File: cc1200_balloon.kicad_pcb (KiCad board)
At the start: 4 copper layers, 50 x 30 mm, 103 parts, among them J101 BATT pads, J201 LoRa ANT pads, J202 SWD+DBG pads, J301 434MHz ANT pads, J401 GNSS ANT, J501 BMV080, Q101 DMG3401LSN-7, U201 Wio-E5, U301 CC1200, U401 AT6558R-5N32, U501 SCD40-D-R2, U502 AS3935-BQFT, U503 BME688, U504 BME688, X301 40MHz, X401 TCXO 26MHz, X402 32.768kHz

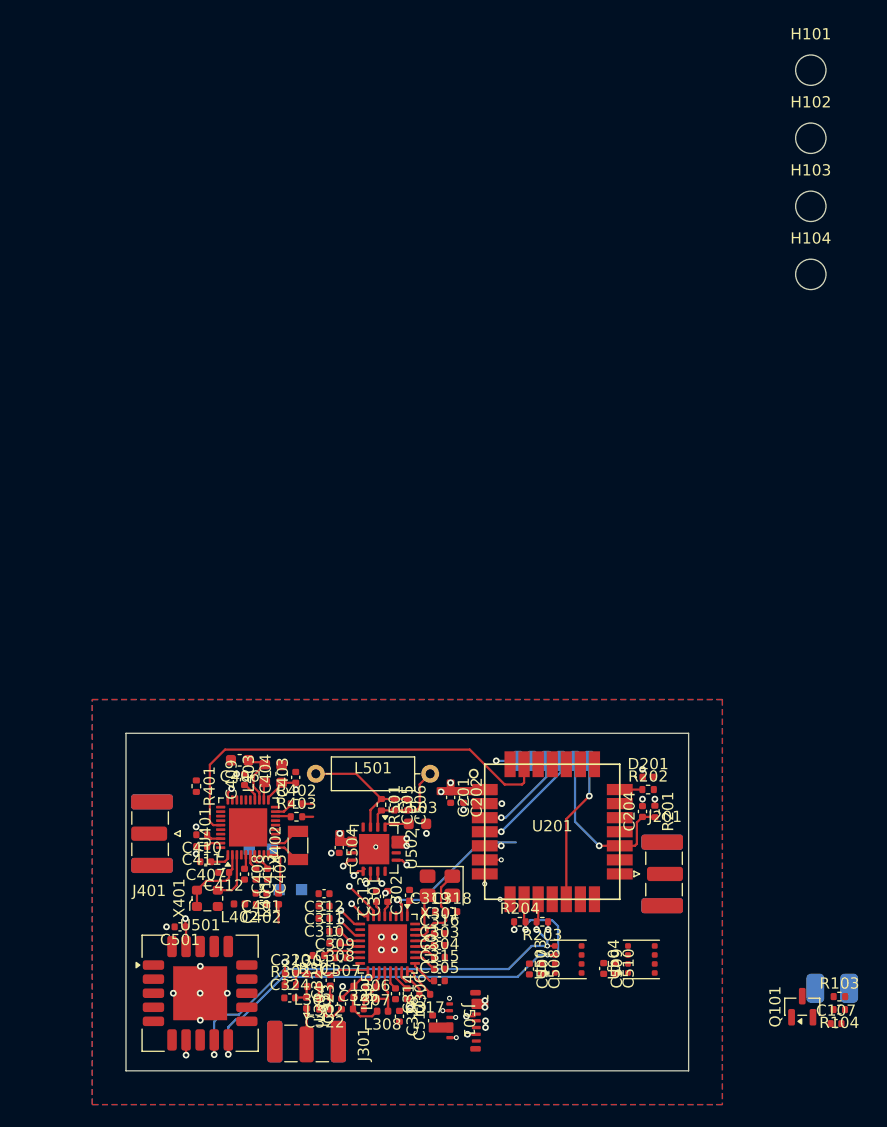
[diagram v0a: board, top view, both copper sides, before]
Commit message: Route, mostly done.
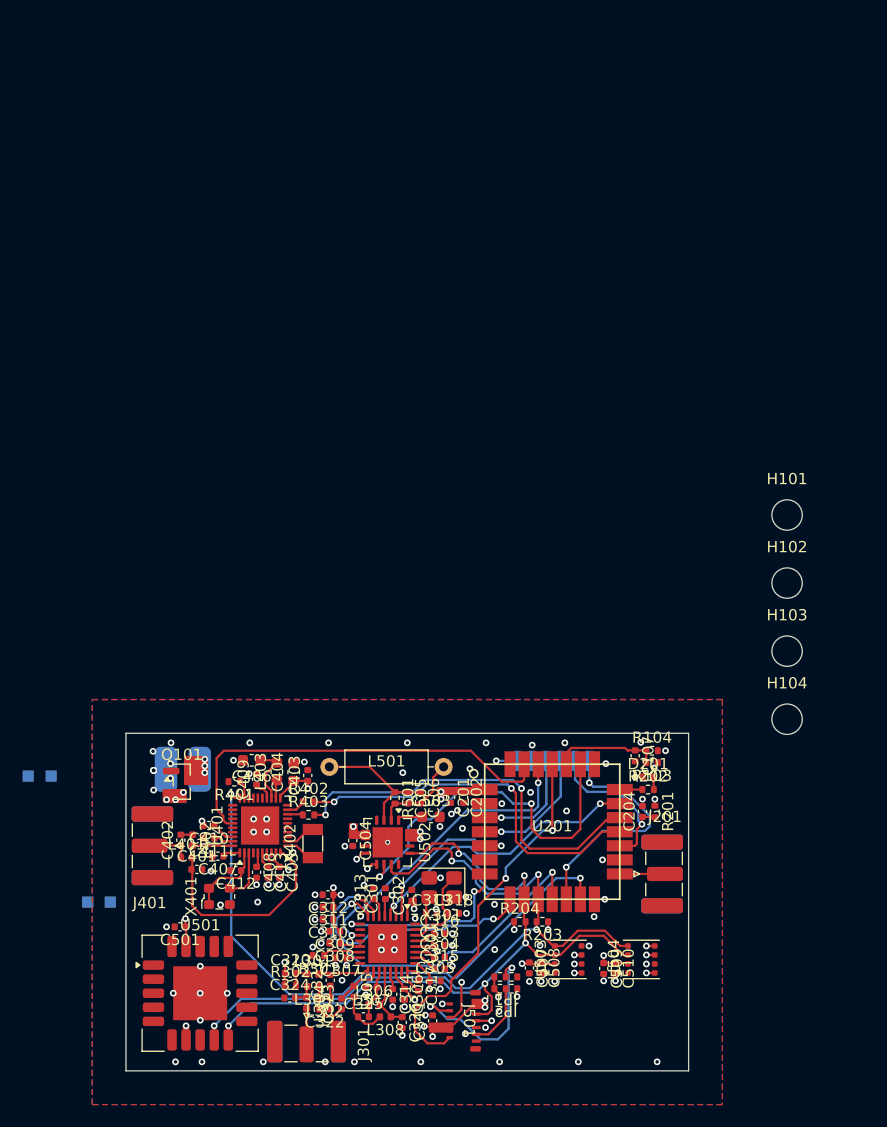
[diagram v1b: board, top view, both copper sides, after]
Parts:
- added JP1: IAB0, cc1200_balloon:Jumper_3_0402, F.Cu at (108.8, 106.7)
- added JP2: IAB1, cc1200_balloon:Jumper_3_0402, F.Cu at (108.8, 107.7)
- moved J101 60.9 mm to (80.0, 88.2)
- moved Q101 58.7 mm to (80.0, 89.3), turned to 0 degrees
- moved H102 39.6 mm to (133.8, 71.7)
- moved H103 39.6 mm to (133.8, 77.7)
- moved H101 39.6 mm to (133.8, 65.6)
- moved H104 39.6 mm to (133.8, 83.8)
- moved C107 29.7 mm to (120.2, 87.0), turned to -90 degrees
- moved R104 28.4 mm to (121.8, 86.5), turned to 0 degrees
- moved R103 26.6 mm to (121.8, 87.6), turned to 180 degrees
- moved TP401 20.7 mm to (66.3, 88.8)
- moved TP402 20.7 mm to (68.3, 88.8)
- moved TP301 17.0 mm to (71.6, 100.0)
- moved TP302 17.0 mm to (73.6, 100.0)
- moved C402 9.17 mm to (79.9, 94.5), turned to 90 degrees
- moved L401 8.96 mm to (80.4, 96.0), turned to 0 degrees
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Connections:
- J501 pad 11: SPI_MISO -> /Sensors/IAB1
- J501 pad 4: PM_CS -> /Sensors/IAB0
- J501 pad 5: SPI_MOSI -> SDA
- J501 pad 6: SPI_SCK -> SCL
- J501 pad 7: GND -> +BATT
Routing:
- net GNSS_ONOFF: track 1.14 -> 53.3 mm, vias 1 -> 2
- net GNSS_RX: track 0.82 -> 35.4 mm, vias 0 -> 2
- net PM_IRQ: track 0.58 -> 33.9 mm, vias 1 -> 2
- net GNSS_TX: track 0.82 -> 33.4 mm, vias 0 -> 2
- net LIGHTNING_IRQ: track 1.24 -> 32.4 mm, vias 1 -> 2
- net SPI_MOSI: track 4.29 -> 34.0 mm
- net SCL: track 43.1 -> 71.2 mm, vias 4 -> 5
- net +BATT: track 33.6 -> 59.1 mm, vias 17 -> 41
- net RADIO_IRQ: track 0.00 -> 25.4 mm, vias 0 -> 2
- net RADIO_CS: track 2.28 -> 27.5 mm, vias 1 -> 2
- net SDA: track 46.4 -> 66.6 mm, vias 4 -> 5
- net SPI_SCK: track 3.33 -> 23.0 mm, vias 3 -> 2
- net /Sensors/IAB0: track 0.00 -> 17.2 mm, vias 0 -> 2
- net /GNSS/GNSS_ANT_BIAS: track 4.31 -> 18.6 mm
- net SPI_MISO: track 3.87 -> 16.5 mm, vias 3 -> 2
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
